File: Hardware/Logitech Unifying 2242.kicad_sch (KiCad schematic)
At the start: 11 parts, among them J1 Bus_M.2_Socket_B, J2 USB, U1 TPS613222ADBV

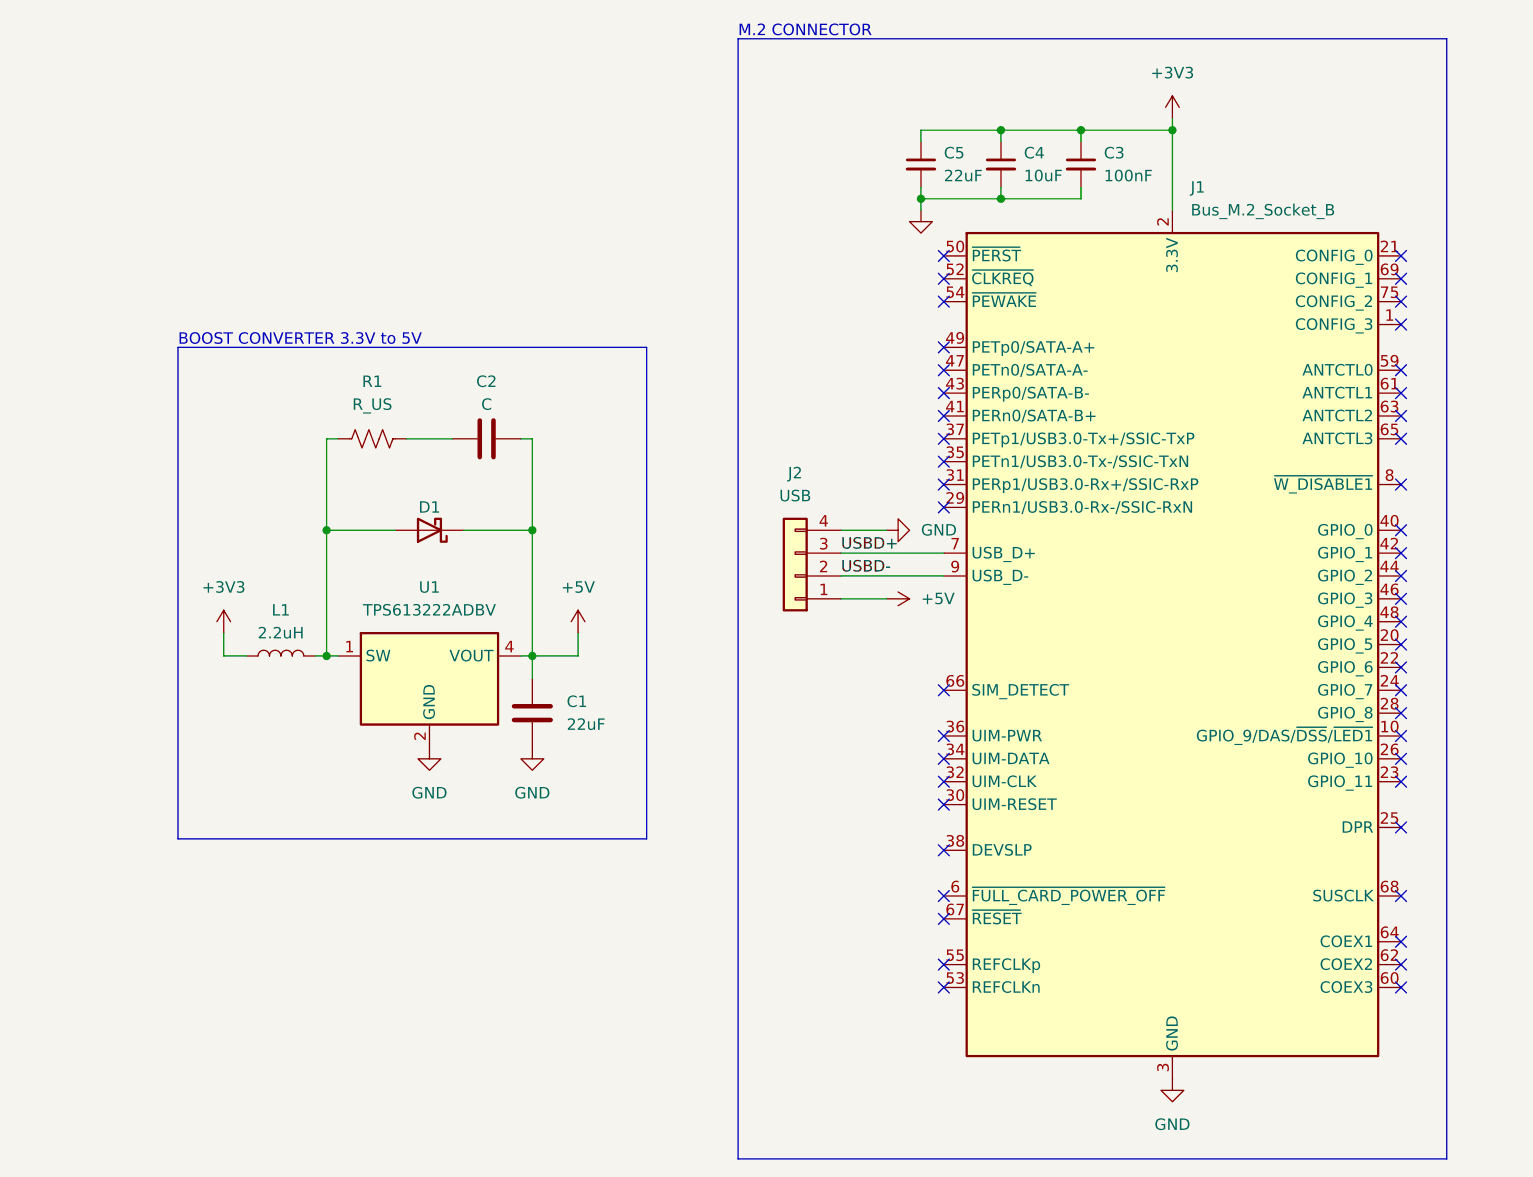
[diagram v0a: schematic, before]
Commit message: Finish layout and routing
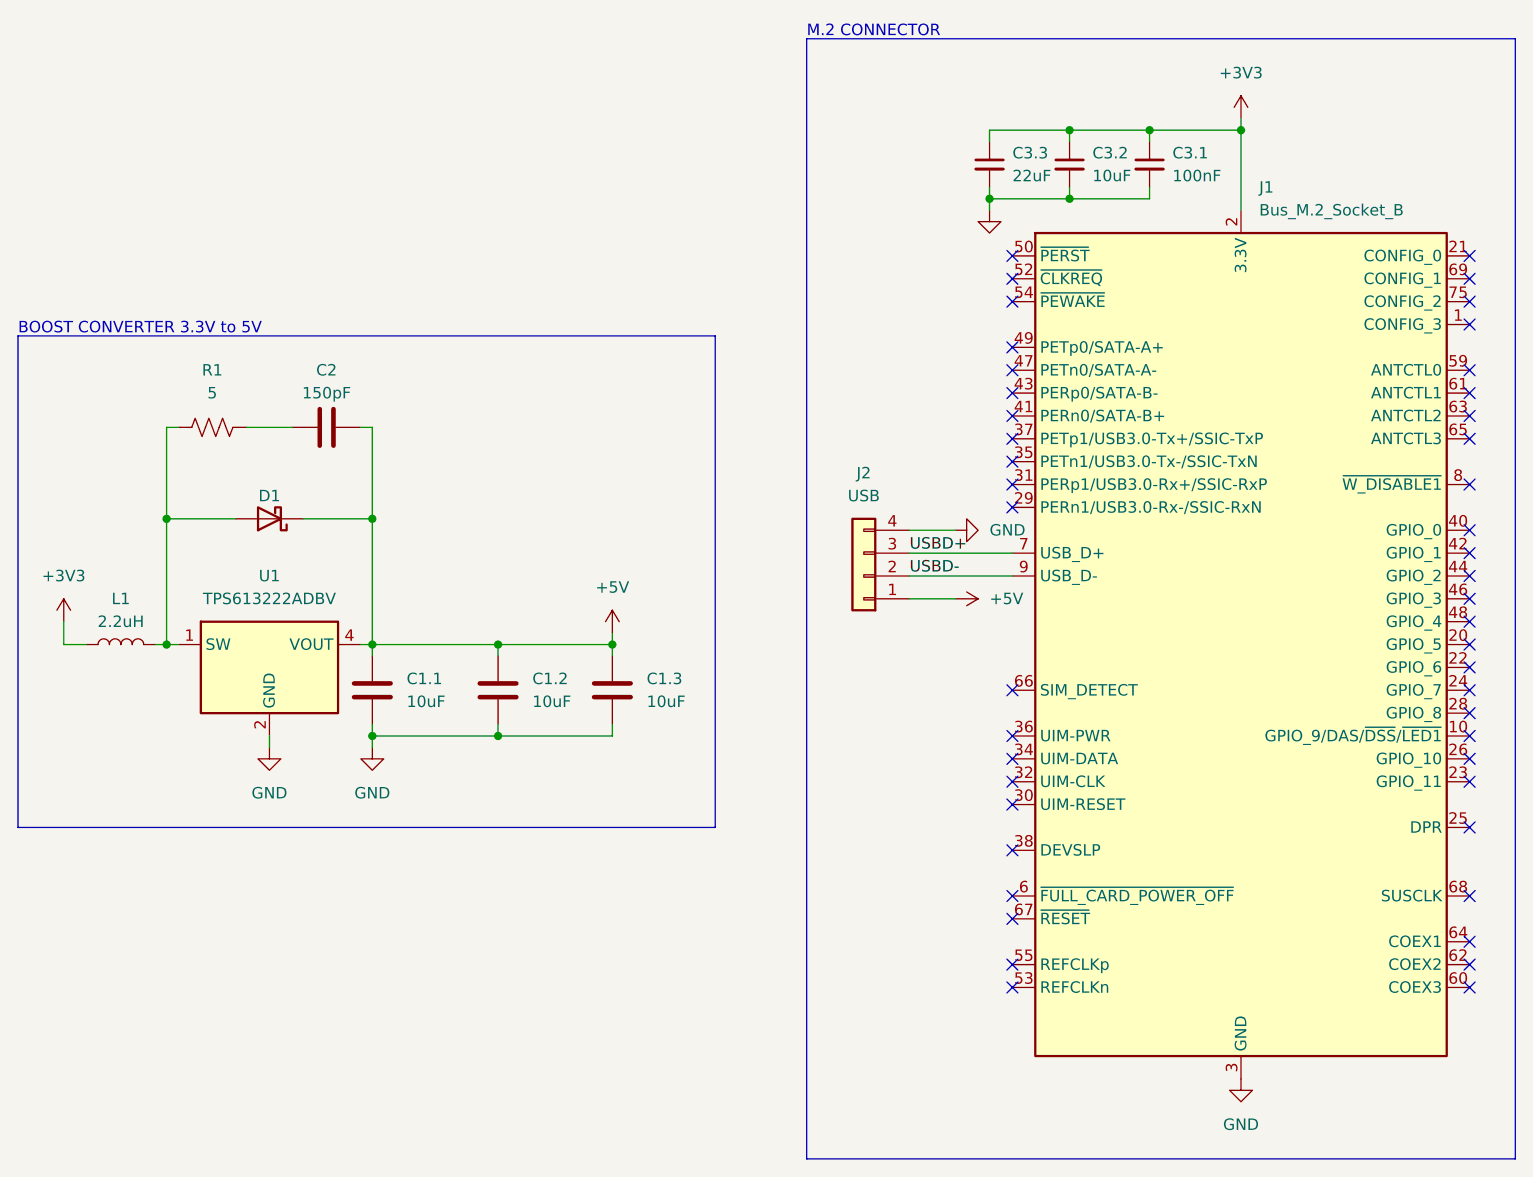
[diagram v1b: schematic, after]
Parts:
- added C1.2, C1.3: 10uF, Capacitor_SMD:C_0805_2012Metric_Pad1.18x1.45mm_HandSolder, symbol Device:C
- C1.1: renamed from C1; value 22uF -> 10uF; footprint (none) -> Capacitor_SMD:C_0805_2012Metric_Pad1.18x1.45mm_HandSolder
- C2: value C -> 150pF; footprint (none) -> Capacitor_SMD:C_0603_1608Metric_Pad1.08x0.95mm_HandSolder
- C3.1: renamed from C3; footprint (none) -> Capacitor_SMD:C_0603_1608Metric_Pad1.08x0.95mm_HandSolder
- C3.2: renamed from C4; footprint (none) -> Capacitor_SMD:C_0805_2012Metric_Pad1.18x1.45mm_HandSolder
- C3.3: renamed from C5; footprint (none) -> Capacitor_SMD:C_0805_2012Metric_Pad1.18x1.45mm_HandSolder
- D1: footprint (none) -> Diode_SMD:D_SMA
- J2: footprint (none) -> Connector_USB:USB_A_TE_292303-7_Horizontal
- L1: footprint (none) -> Inductor_SMD:L_1008_2520Metric_Pad1.43x2.20mm_HandSolder
- R1: value R_US -> 5; footprint (none) -> Resistor_SMD:R_0805_2012Metric_Pad1.20x1.40mm_HandSolder
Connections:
- net +5V: now also C1.2.1, C1.3.1
- net GND: now also C1.2.2, C1.3.2
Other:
- moved on the sheet: C1.1, C2, C3.1, C3.2, C3.3, D1, J1, J2, L1, R1, U1

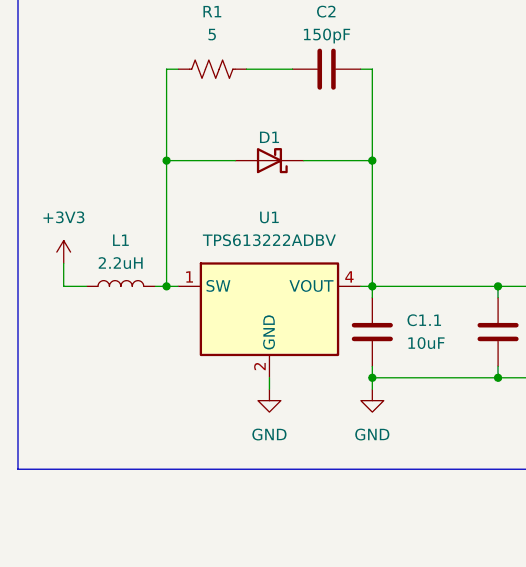
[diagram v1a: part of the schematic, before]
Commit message: Update M.2 footprints
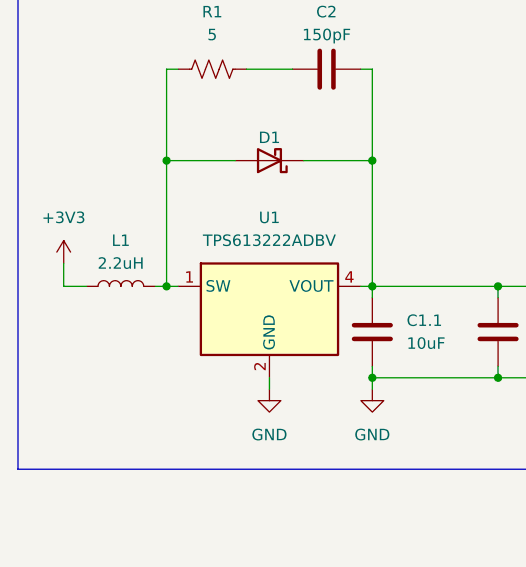
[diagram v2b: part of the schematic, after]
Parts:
- J1: footprint Connector_OTHER:M.2-2242-B+M-KEY -> Connector_OTHER:M.2-2242-B+M-KEY_USB-ONLY
